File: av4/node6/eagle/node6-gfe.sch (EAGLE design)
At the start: 18 parts, among them J1 MICROSDMOL500873, J15 Auxiliary Header, J2 ROCKETNET-CONNECTOR-16M, U1 DP83630/LLP, U2 STM32F407V_NODE6/LQFP100

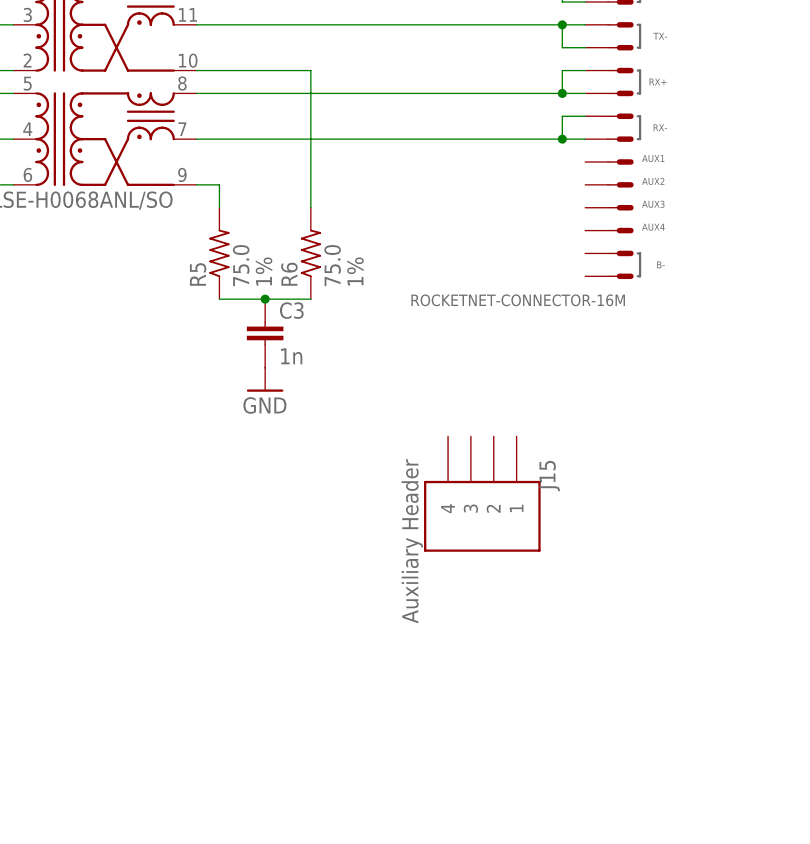
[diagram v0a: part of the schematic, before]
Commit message: node6: hooked up aux connector to rocketnet
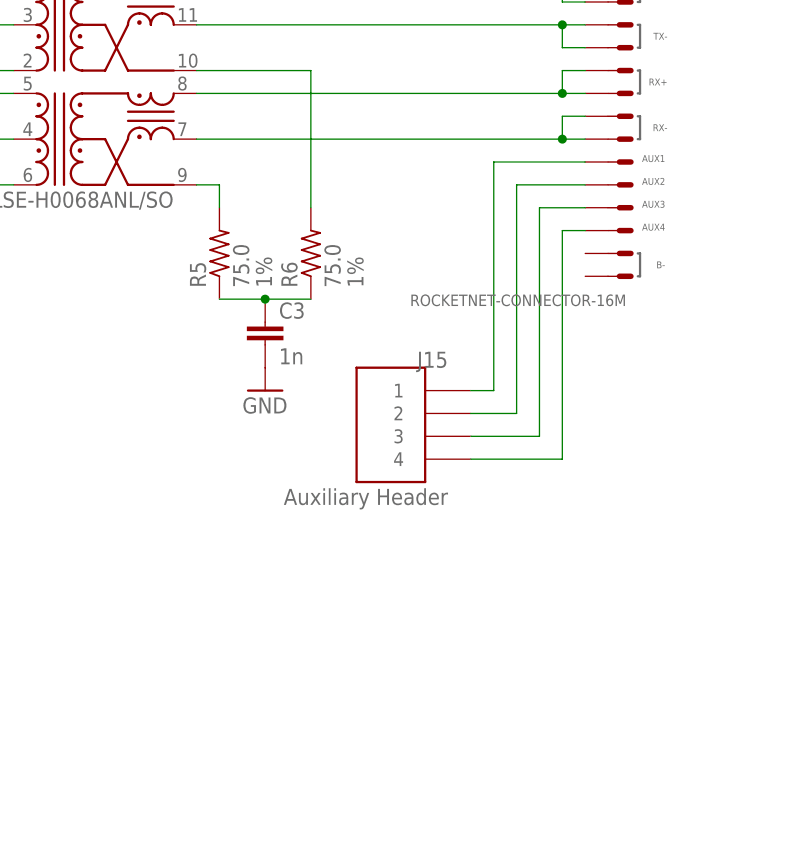
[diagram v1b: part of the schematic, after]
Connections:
- new net N$21: J15.1, J2.AUX1
- new net N$22: J15.2, J2.AUX2
- new net N$23: J15.3, J2.AUX3
- new net N$24: J15.4, J2.AUX4
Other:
- moved on the sheet: J15
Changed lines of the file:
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@@
 </instance>
 <instance part="J2" gate="G$1" x="370.84" y="208.28" rot="MR0"/>
-<instance part="J15" gate="J" x="353.06" y="162.56" rot="R270"/>
+<instance part="J15" gate="J" x="345.44" y="170.18" rot="MR0"/>
 <instance part="C1" gate="CE" x="246.38" y="182.88"/>
 <instance part="L1" gate="G$1" x="312.42" y="210.82"/>
@@
 </segment>
 </net>
+<net name="N$21" class="0">
+<segment>
+<pinref part="J2" gate="G$1" pin="AUX1"/>
+<wire x1="365.76" y1="200.66" x2="355.6" y2="200.66" width="0.1524" layer="91"/>
+<wire x1="355.6" y1="200.66" x2="355.6" y2="175.26" width="0.1524" layer="91"/>
+<pinref part="J15" gate="J" pin="1"/>
+<wire x1="355.6" y1="175.26" x2="353.06" y2="175.26" width="0.1524" layer="91"/>
+</segment>
+</net>
+<net name="N$22" class="0">
+<segment>
+<pinref part="J15" gate="J" pin="2"/>
+<wire x1="353.06" y1="172.72" x2="358.14" y2="172.72" width="0.1524" layer="91"/>
+<wire x1="358.14" y1="172.72" x2="358.14" y2="198.12" width="0.1524" layer="91"/>
+<pinref part="J2" gate="G$1" pin="AUX2"/>
+<wire x1="358.14" y1="198.12" x2="365.76" y2="198.12" width="0.1524" layer="91"/>
+</segment>
+</net>
+<net name="N$23" class="0">
+<segment>
+<pinref part="J15" gate="J" pin="3"/>
+<wire x1="353.06" y1="170.18" x2="360.68" y2="170.18" width="0.1524" layer="91"/>
+<wire x1="360.68" y1="170.18" x2="360.68" y2="195.58" width="0.1524" layer="91"/>
+<pinref part="J2" gate="G$1" pin="AUX3"/>
+<wire x1="360.68" y1="195.58" x2="365.76" y2="195.58" width="0.1524" layer="91"/>
+</segment>
+</net>
+<net name="N$24" class="0">
+<segment>
+<pinref part="J15" gate="J" pin="4"/>
+<wire x1="353.06" y1="167.64" x2="363.22" y2="167.64" width="0.1524" layer="91"/>
+<wire x1="363.22" y1="167.64" x2="363.22" y2="193.04" width="0.1524" layer="91"/>
+<pinref part="J2" gate="G$1" pin="AUX4"/>
+<wire x1="363.22" y1="193.04" x2="365.76" y2="193.04" width="0.1524" layer="91"/>
+</segment>
+</net>

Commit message: node6: finished sd card symbol. added sd and power supply front end to schematic
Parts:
- removed J1: MICROSDMOL500873, connector:MICROSDMOL500873
- added C2000: 100n 50V, rcl_custom:C-EU0603-B-NOSILK
- added C2001: 22u 50V, rcl:CPOL-USD/7343-31R
- added C2002: 330n 50V, rcl_custom:C-EU0603-B-NOSILK
- added C2003: 2.7u, rcl_custom:C-EU0603-B-NOSILK
- added C2004: 15n, rcl_custom:C-EU0603-B-NOSILK
- added C2011: 10n 50V, rcl_custom:C-EU0603-B-NOSILK
- added D2001: CDSU101A, psas_eagle_library:DIODE_SILICON-0603
- added F2000: 2.0A Fast, custom:FUSE1206
- added J3: MICROSD-7T-DET504077, sd_card:MICROSD-7T-DET504077
- added L2000: CMS1, choke:COIL_CMS1
- added Q2000, Q2002: PMV45EN, Tova:PMV45EN
- added Q2001: Si7309DN, 0kaz:P-MOS_SI7123DN
- added R2000: 100k, rcl_custom:R-US_0603-B-NOSILK
- added R2001: 61.9k, rcl_custom:R-US_0603-B-NOSILK
- added R2002, R2012: 10k, rcl_custom:R-US_0603-B-NOSILK
- added R2003: .033, rcl_custom:R-US_0805-B-NOSILK
- added R2004: 1k, rcl_custom:R-US_0603-B-NOSILK
- added R2005: 34.0k 1%, rcl_custom:R-US_0603-B-NOSILK
- added R2006: 10k 1%, rcl_custom:R-US_0603-B-NOSILK
- added TVS2000: TVS_SMB, 0kaz:TVS_SMB
- added U2000: MAX5902AAEUT, node4:IC_MAX5902
- added U2001: TLV3012AIDBVT, node4:IC_TLV3012
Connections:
- net N$1 renamed RNET_TX-
- net N$2 renamed RNET_RX+
- net N$21 renamed RNET_AUX1
- net N$22 renamed RNET_AUX2
- net N$23 renamed RNET_AUX3
- net N$24 renamed RNET_AUX4
- net N$4 renamed RNET_RX-
- net N$6 renamed RNET_TX+
- new net BIN: F2000.1, L2000.3
- new net CHASSIS: C2000.1, R2000.1
- new net IN+: C2004.1, R2005.1, R2006.2, U2001.IN+
- new net MAX_UVLO: Q2000.D, R2001.1, R2002.2, U2000.ON_OFF/
- new net N$334: Q2001.D, R2003.1
- new net N_DRAIN: Q2002.D, R2004.1, U2000.DRAIN
- new net N_GATE: C2004.2, Q2002.G, U2001.OUT
- new net PORT1.0/GPIO_SPS_DISABLE: Q2000.G, R2012.2
- new net PORT1.1/GPIO_SPS_V-IN_GOOD: U2000.PGOOD/
- new net P_GATE: Q2001.G, U2000.GATE
- new net REF: U2001.IN-, U2001.REF
- new net RNET_B+: J2.B+@1, J2.B+@2, L2000.4
- new net RNET_B-: J2.B-@1, J2.B-@2, L2000.1
- new net SPS_OUT: D2001.ANODE, R2005.2
- new net V+1: C2003.2, D2001.CATHODE, U2001.V+
- new net VIN: R2003.2, R2004.2
- new net V_FUSED: C2001.+, C2002.2, C2011.2, F2000.2, Q2001.S, R2001.2, TVS2000.CATHODE, U2000.VS
- net GND: now also C2000.2, C2001.-, C2002.1, C2003.1, C2011.1, J3G$2.TAB, J3G$3.TAB, J3G$4.TAB, J3G$5.TAB, J3G$6.TAB, J3G$7.TAB, J3G$8.TAB, L2000.2, Q2000.S, Q2002.S, R2000.2, R2002.1, R2006.1, R2012.1, TVS2000.ANODE, U1.ANAVSS, U1.CD_VSS, U1.DAP, U1.IO_CORE_VSS, U1.IO_VSS, U2000.GND, U2001.V-
- net SD_CLK: now also J3G$1.CLK/SCLK, U2.PC12/SDIO_CK; no longer J1G$1.CLK/SCLK
- net SD_CMD: now also J3G$1.CMD/DI, U2.PD2/SDIO_CMD; no longer J1G$1.CMD/DI
- net SD_DAT0: now also J3G$1.DAT0/DO, U2.PC8/SDIO_D0; no longer J1G$1.DAT0/DO
- net SD_DAT1: now also J3G$1.DAT1/RSV, U2.PC9/SDIO_D1; no longer J1G$1.DAT1/RSV
- net SD_DAT2: now also J3G$1.DAT2/RSV, U2.PC10/SDIO_D2; no longer J1G$1.DAT2/RSV
- net SD_DAT3: now also J3G$1.CD/DAT3/!CS, U2.PC11/SDIO_D3; no longer J1G$1.CD/DAT3/!CS
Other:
- note added: "18.2K if SPS=3.3V"
- note added: "REQUIRES LPC PULL-UP"
- note added: "Rcb"
- note added: "SPS_OUT Over Voltage Sense"
- note removed: "todo placeholder package"

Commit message: node6: added ltm8023 power supply
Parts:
- added C103: 2.2u/40V, rcl_custom:C-EU0603-B-NOSILK
- added C104: 2.2u, rcl_custom:C-EU0603-B-NOSILK
- added J13: PGOOD Jumper, headers:1.27MM_HDR_2X12X1
- added LED22: GREEN, led:LEDCHIPLED_0603
- added R128: 750, rcl_custom:R-US_0402-B-NOSILK
- added R131: 10k, rcl_custom:R-US_0402-B-NOSILK
- added R73: 154k, rcl_custom:R-US_0402-B-NOSILK
- added R74: 49.9k, rcl_custom:R-US_0402-B-NOSILK
- added U5: LTM8023, RNH_LTM8023:LTM8023
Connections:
- removed net VIN: R2003.2, R2004.2
- new net +18V: C103.1, R2003.2, R2004.2, U5.RUN/SS, U5.VIN
- new net +3V3: C104.1, R128.1, U5.VOUT
- new net N$116: R73.2, U5.ADJ
- new net N$117: R74.2, U5.RT
- new net N$29: J13.2, LED22.A, U5.PGOOD
- new net N$30: J13.1, R128.2
- new net N$37: U5.AUX, U5.BIAS
- new net SD_DETECT: J3G$9.DET
- new net SYNC: R131.1, U5.SYNC
- net GND: now also C103.2, C104.2, LED22.C, R131.2, R73.1, R74.1, U5.GND
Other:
- note added: "+72V Hot Swap Controller"
- note added: "3.3V Switching Supply"
- note added: "TODO: Sync, power good, etc."
- moved on the sheet: C1, C2, C2003, C2004, C3, C4, C5, J15, J2, L1, R1, R2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

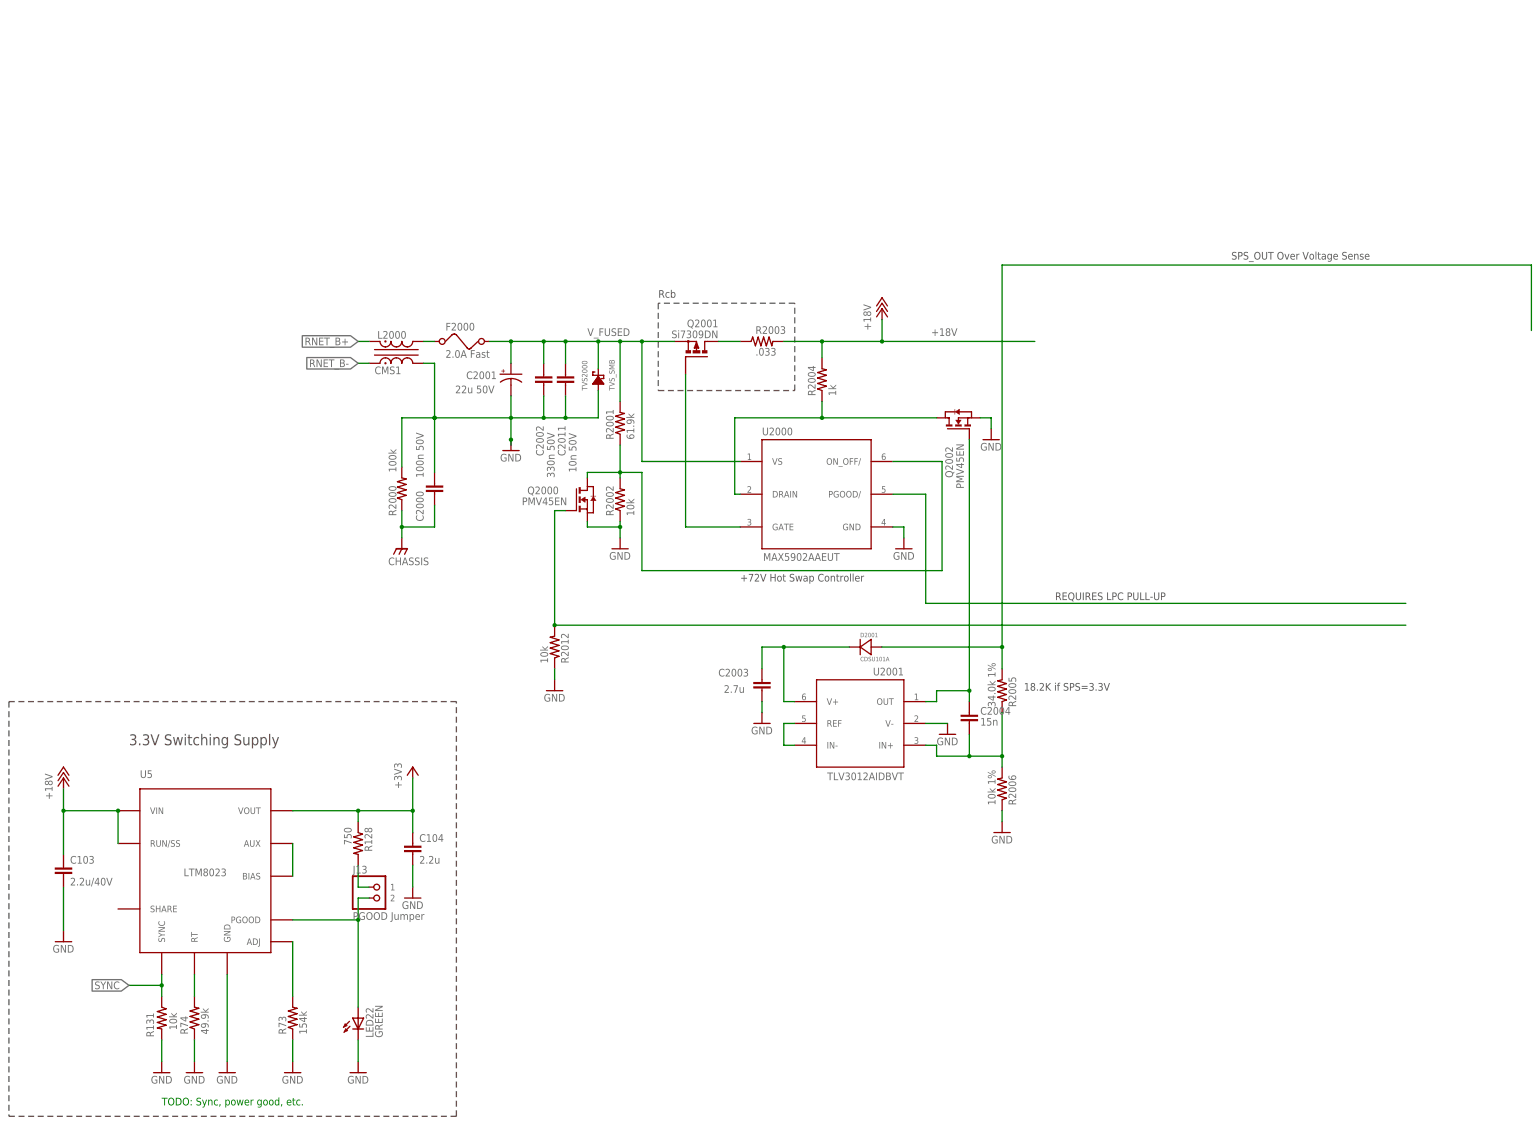
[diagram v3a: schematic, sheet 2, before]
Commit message: node6: new regulator library, added ltc3586, primary switcher output +5
moving toward ltc3586 as main switching chip to generate 3.3 and 5, buck
regulators available to generate other supplies if needed in other
projects.
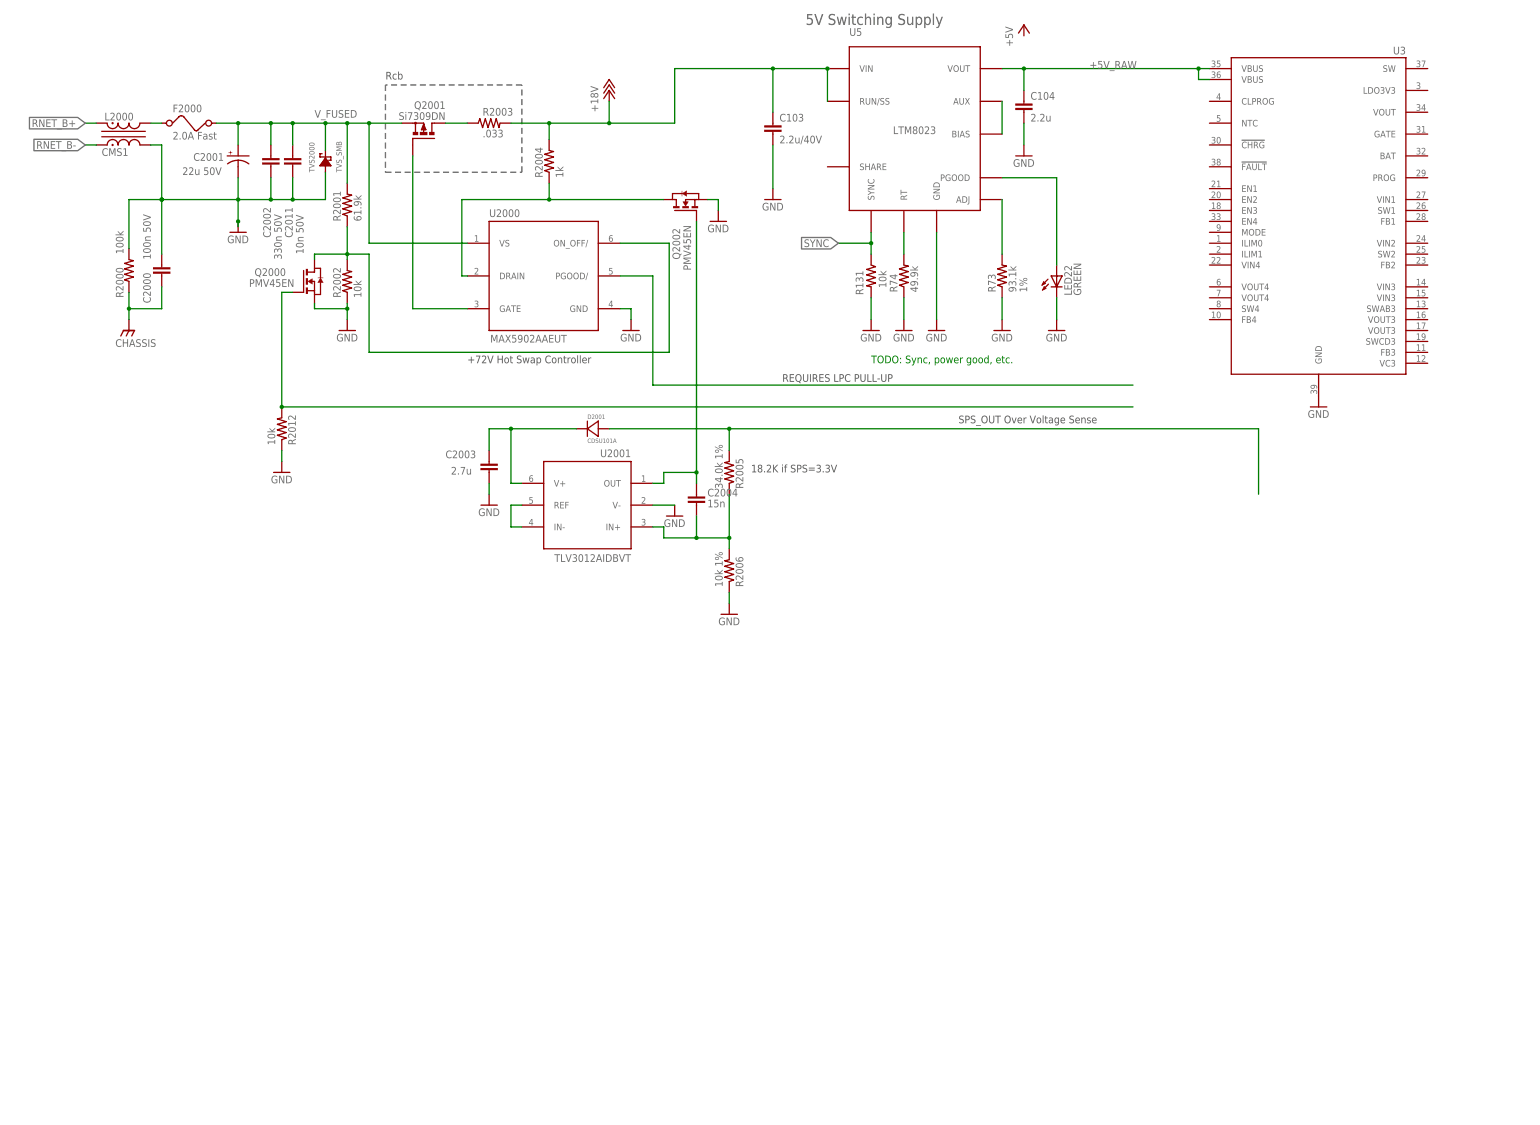
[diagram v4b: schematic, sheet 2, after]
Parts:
- removed J13: PGOOD Jumper, headers:1.27MM_HDR_2X12X1
- removed R128: 750, rcl_custom:R-US_0402-B-NOSILK
- added U3: LTC3586, regulator:LTC3586
- R73: value 154k -> 93.1k; TOLERANCE (none) -> 1%
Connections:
- removed net +3V3: C104.1, R128.1, U5.VOUT
- removed net N$29: J13.2, LED22.A, U5.PGOOD
- removed net N$30: J13.1, R128.2
- new net +5V_RAW: C104.1, U3.VBUS@1, U3.VBUS@2, U5.VOUT
- new net PGOOD_5V: LED22.A, U5.PGOOD
- net GND: now also U3.GND
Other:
- note added: "5V Switching Supply"
- note removed: "3.3V Switching Supply"
- moved on the sheet: C103, C104, C2000, C2001, C2002, C2003, C2004, C2011, D2001, F2000, L2000, LED22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
